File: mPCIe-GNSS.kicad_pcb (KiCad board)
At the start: 2 copper layers, 30 x 51 mm, 23 parts, among them J1 1PPS, J2 ANT, Q1 DTC143Z, Q2 DTA043T, U1 FT234XD-T

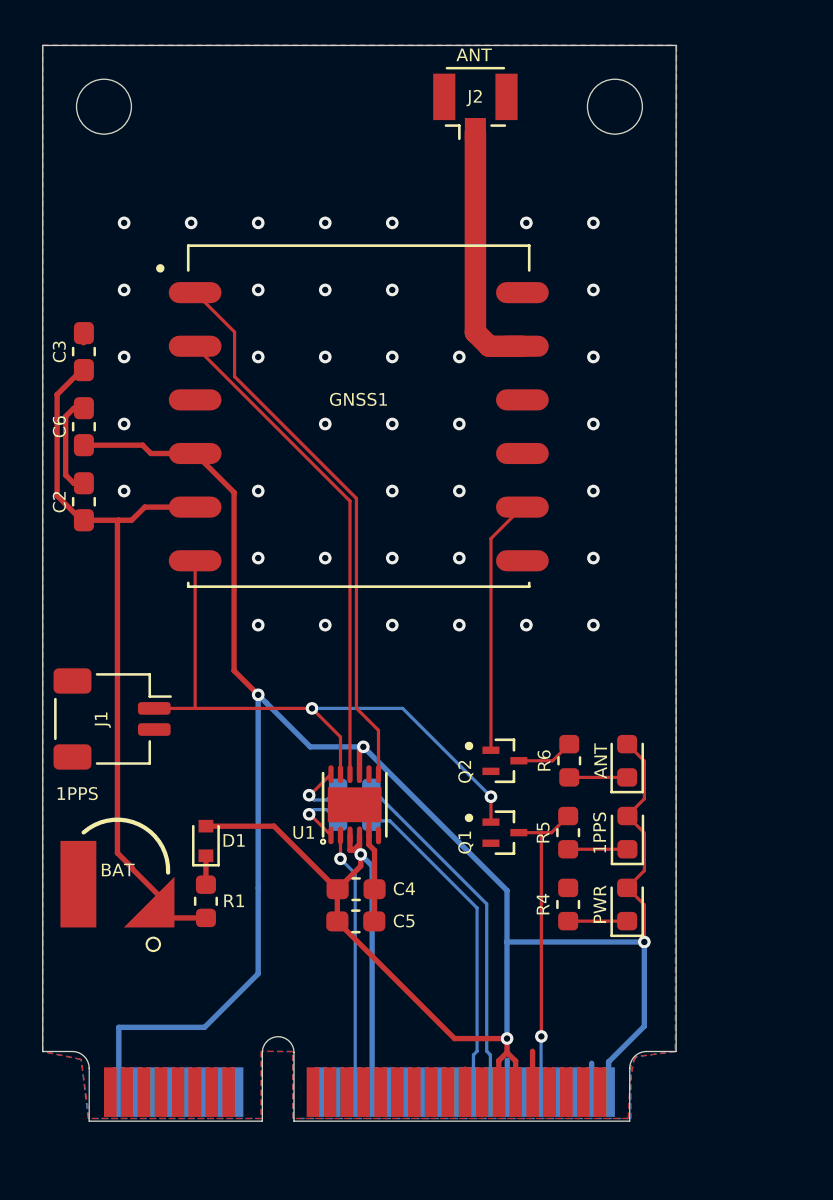
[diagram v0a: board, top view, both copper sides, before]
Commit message: version 0.3
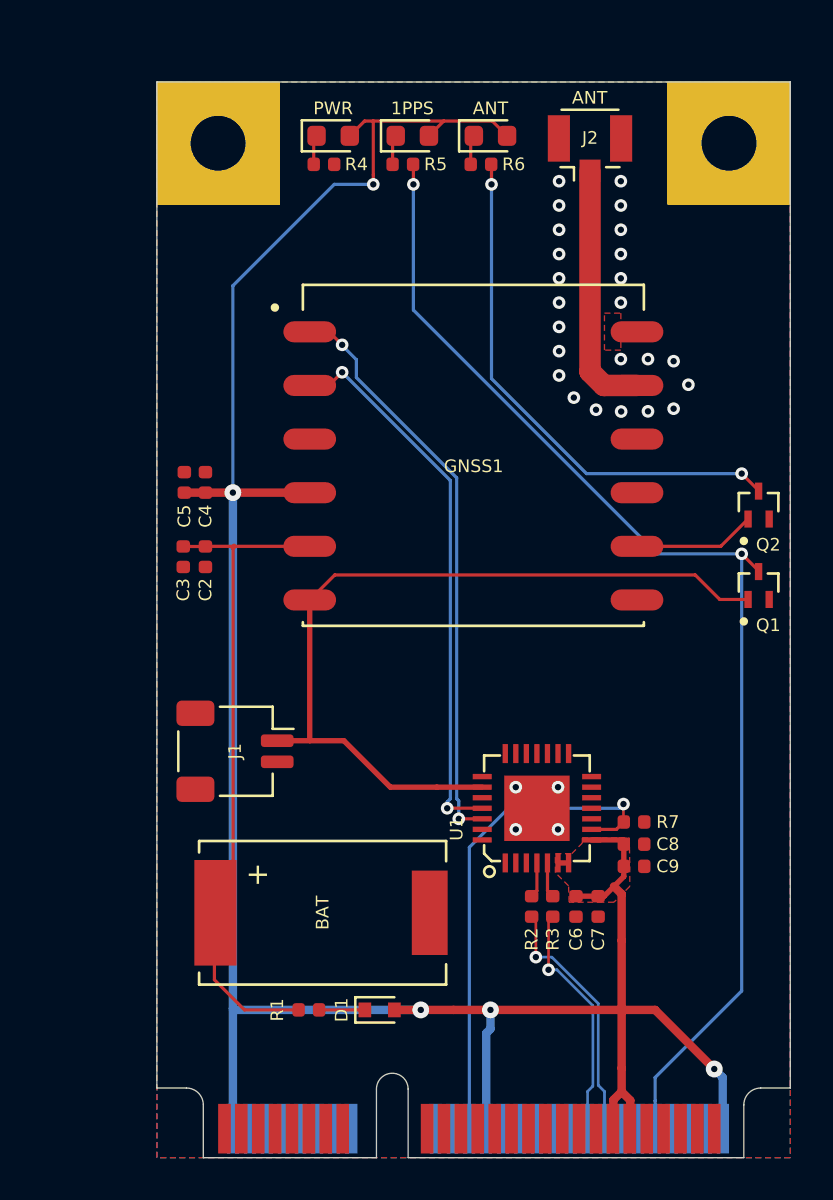
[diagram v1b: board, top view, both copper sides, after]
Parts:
- added C7: 4.7uF, Capacitor_SMD:C_0402_1005Metric, F.Cu at (143.1, 118.1)
- added C8: 100nF, Capacitor_SMD:C_0402_1005Metric, F.Cu at (144.8, 115.2)
- added C9: 1uF, Capacitor_SMD:C_0402_1005Metric, F.Cu at (144.8, 116.2)
- added R7: 4.7K, Resistor_SMD:R_0402_1005Metric, F.Cu at (144.8, 114.1)
- C1: value XH414HG -> DSK-3R3H224U-HL; footprint L80:CAP_XH414H-IV01E -> 1 My Footprints:CAP_DSK-3R3H224U-HL
- C2, C3, C4, C5, C6: footprint Capacitor_SMD:C_0603_1608Metric_Pad1.05x0.95mm_HandSolder -> Capacitor_SMD:C_0402_1005Metric
- GNSS1: footprint L80:XCVR_LC86L -> 1 My Footprints:XCVR_LC86L
- J1: footprint Connector_JST:JST_SH_SM02B-SRSS-TB_1x02-1MP_P1.00mm_Horizontal -> 1 My Footprints:JST_SH_SM02B-SRSS-TB_1x02-1MP_P1.00mm_Horizontal_3D
- LED1, LED2, LED3: footprint LED_SMD:LED_0603_1608Metric -> 1 My Footprints:LED_0603_1608Metric_SnapModel
- PC1: footprint mini-PCIe Cards:mini-PCIe_F1_Full -> 1 My Footprints:mini-PCIe_F1_Full_v600
- Q1, Q2: footprint L80:Q-EMT3 -> 1 My Footprints:Q_EMT3F
- R1: footprint Resistor_SMD:R_0603_1608Metric -> Resistor_SMD:R_0402_1005Metric
- R2, R3: value 27R -> 33R; footprint Resistor_SMD:R_0603_1608Metric -> Resistor_SMD:R_0402_1005Metric; moved to F.Cu
- R4: value 1K -> 51R; footprint Resistor_SMD:R_0603_1608Metric -> Resistor_SMD:R_0402_1005Metric
- R5, R6: value 1K -> 220R; footprint Resistor_SMD:R_0603_1608Metric -> Resistor_SMD:R_0402_1005Metric
- U1: value FT234XD-T -> CP2102N-A01-GQFN28; footprint L80:SON45P300X300X80-13N -> 1 My Footprints:QFN28G_0.5-5X5MM
- moved LED1 39.0 mm to (130.6, 81.6), turned to 0 degrees
- moved R4 36.9 mm to (130.1, 83.0), turned to 0 degrees
- moved LED2 34.5 mm to (134.3, 81.6), turned to 0 degrees
- moved R5 32.6 mm to (133.8, 83.0), turned to 0 degrees
- moved C6 32.5 mm to (142.1, 118.1)
- moved LED3 30.3 mm to (138.0, 81.6), turned to 0 degrees
- moved R6 28.6 mm to (137.6, 83.0), turned to 0 degrees
- moved C5 22.3 mm to (123.5, 98.0), turned to 270 degrees
- moved C4 20.5 mm to (124.5, 98.0), turned to 90 degrees
- moved Q2 17.1 mm to (150.7, 99.1), turned to 90 degrees
- moved Q1 16.8 mm to (150.7, 102.9), turned to 90 degrees
- moved D1 11.5 mm to (132.8, 123.0), turned to 0 degrees
- moved C3 10.8 mm to (123.5, 101.5), turned to 270 degrees
- moved R3 10.2 mm to (140.9, 118.1), turned to 270 degrees
- moved R2 10.1 mm to (139.9, 118.1), turned to 90 degrees
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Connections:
- net +BATT renamed /VBAT
- net /LED_WLAN renamed /~LED_WLAN
- C6 pad 1: +3.3V -> GND
- C6 pad 2: GND -> +3.3V
- GNSS1 pad 10: Net-(GNSS1-Pad10) -> (no net)
- GNSS1 pad 7: Net-(GNSS1-Pad7) -> (no net)
- GNSS1 pad 9: Net-(GNSS1-Pad9) -> (no net)
- PC1 pad 1: Net-(PC1-Pad1) -> (no net)
- PC1 pad 10: Net-(PC1-Pad10) -> (no net)
- PC1 pad 11: Net-(PC1-Pad11) -> (no net)
- PC1 pad 12: Net-(PC1-Pad12) -> (no net)
- PC1 pad 13: Net-(PC1-Pad13) -> (no net)
- PC1 pad 14: Net-(PC1-Pad14) -> (no net)
- PC1 pad 16: Net-(PC1-Pad16) -> (no net)
- PC1 pad 17: Net-(PC1-Pad17) -> (no net)
- PC1 pad 19: Net-(PC1-Pad19) -> (no net)
- PC1 pad 20: Net-(PC1-Pad20) -> (no net)
- PC1 pad 22: /RESET -> /~RESET
- PC1 pad 23: Net-(PC1-Pad23) -> (no net)
- PC1 pad 25: Net-(PC1-Pad25) -> (no net)
- PC1 pad 28: Net-(PC1-Pad28) -> (no net)
- PC1 pad 3: Net-(PC1-Pad3) -> (no net)
- PC1 pad 30: Net-(PC1-Pad30) -> (no net)
- PC1 pad 31: Net-(PC1-Pad31) -> (no net)
- PC1 pad 32: Net-(PC1-Pad32) -> (no net)
- PC1 pad 33: Net-(PC1-Pad33) -> (no net)
- PC1 pad 42: Net-(PC1-Pad42) -> (no net)
- PC1 pad 45: Net-(PC1-Pad45) -> (no net)
- PC1 pad 46: Net-(PC1-Pad46) -> (no net)
- PC1 pad 47: Net-(PC1-Pad47) -> (no net)
- PC1 pad 48: Net-(PC1-Pad48) -> (no net)
- PC1 pad 49: Net-(PC1-Pad49) -> (no net)
- PC1 pad 5: Net-(PC1-Pad5) -> (no net)
- PC1 pad 51: Net-(PC1-Pad51) -> (no net)
- PC1 pad 6: Net-(PC1-Pad6) -> (no net)
- PC1 pad 7: Net-(PC1-Pad7) -> (no net)
- PC1 pad 8: Net-(PC1-Pad8) -> (no net)
- R2 pad 1: /FT_D+ -> /USB_D+
- R2 pad 2: /USB_D+ -> /U232_D+
- R3 pad 1: /USB_D- -> /U232_D-
- R3 pad 2: /FT_D- -> /USB_D-
- U1 pad 1: /FT_D- -> (no net)
- U1 pad 10: /GPS_TX -> (no net)
- U1 pad 11: /1PPS -> (no net)
- U1 pad 12: /FT_D+ -> (no net)
- U1 pad 13: GND -> (no net)
- U1 pad 2: /RESET -> (no net)
- U1 pad 3: +3.3V -> GND
- U1 pad 4: +3.3V -> /U232_D+
- U1 pad 5: GND -> /U232_D-
- U1 pad 6: Net-(U1-Pad6) -> +3.3V
- U1 pad 7: /GPS_RX -> +3.3V
- U1 pad 8: Net-(U1-Pad8) -> +3.3V
- U1 pad 9: +3.3V -> /~RESET
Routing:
- net /~LED_WLAN: track 15.0 -> 57.6 mm, vias 1 -> 2
- net /~RESET: track 0.00 -> 24.0 mm, vias 0 -> 1
- net Net-(Q2-Pad3): track 2.71 -> 25.0 mm, vias 0 -> 2
- net GND: track 17.5 -> 1.51 mm, vias 39 -> 28
- net /RESET: track 12.5 -> 0.00 mm, vias 1 -> 0
- net +3.3V: track 131.5 -> 121.3 mm
- net /1PPS: track 29.6 -> 39.0 mm, vias 2 -> 0
- net /AADET_N: track 12.1 -> 5.80 mm
- net /USB_D+: track 17.4 -> 11.9 mm, vias 0 -> 1
- net /USB_D-: track 15.5 -> 11.3 mm, vias 0 -> 1
- net /VBAT: track 35.6 -> 31.5 mm
- net /FT_D-: track 3.51 -> 0.00 mm, vias 1 -> 0
- net /FT_D+: track 3.51 -> 0.00 mm, vias 1 -> 0
- net /GPS_TX: track 23.3 -> 26.3 mm, vias 0 -> 2
- net /U232_D-: track 0.00 -> 1.68 mm
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- added copper zone on F.Cu, net +3.3V
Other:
- net class Default: clearance 0.1524 -> 0.127; trace_width 0.1524 -> 0.127
- net class GNSS Antenna removed
- net class GPS RF added: clearance 0.23093, trace_width 1.02, via_dia 0.6, via_drill 0.3
- net class Power: clearance 0.1524 -> 0.127; via_dia 0.6 -> 0.8
- net class USB Data: clearance 0.1524 -> 0.127; trace_width 0.1524 -> 0.127
- rule pad_to_mask_clearance: 0.05 -> 0
- rule trace_clearance: 0.1524 -> 0.127
- rule trace_min: 0.1524 -> 0.127
